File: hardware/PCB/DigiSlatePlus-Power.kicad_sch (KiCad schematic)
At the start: 38 parts, among them J3 +8-24 Volt, J4 Battery, J5 Mains, Q3 FS8205A, U21 LM2596S-ADJ, U22 DW01A, U23 TP4056, U24 KA78M05_TO252, U25 LD1117S33TR_SOT223

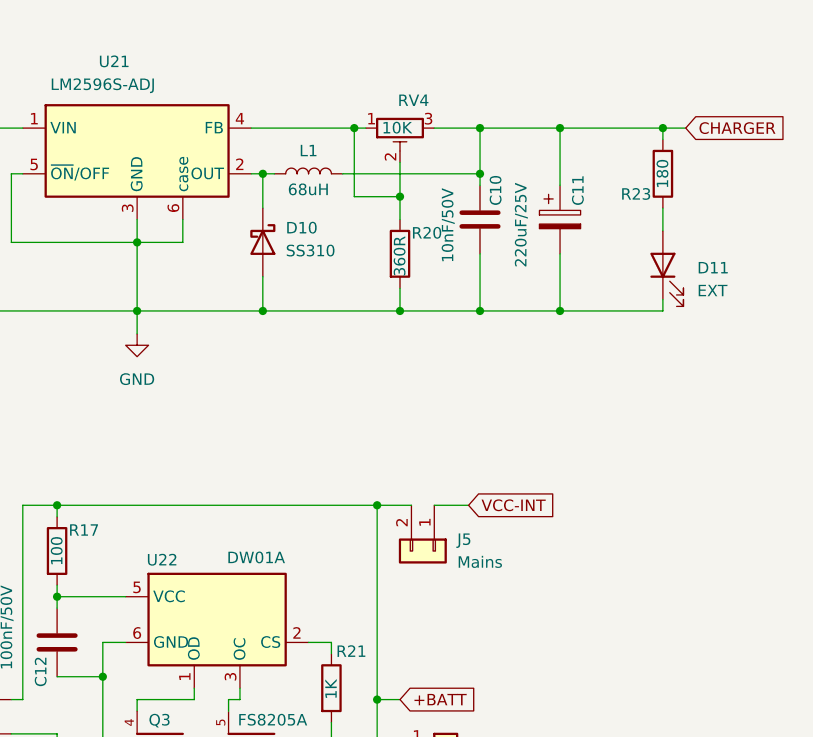
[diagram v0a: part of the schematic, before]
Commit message: final 1.0 board version
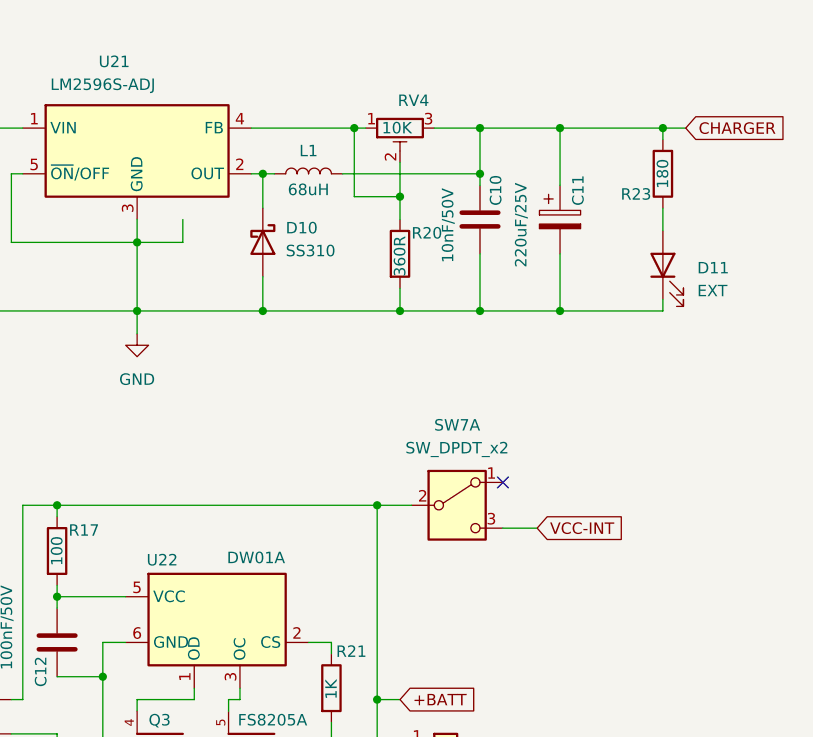
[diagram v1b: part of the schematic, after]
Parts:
- removed J5: Mains, Connector_JST:JST_XH_B2B-XH-AM_1x02_P2.50mm_Vertical, symbol Connector_Generic:Conn_01x02
- added SW7: SW_DPDT_x2, Button_Switch_THT:SW_Slide_SPDT_Angled_CK_OS102011MA1Q, symbol Switch:SW_DPDT_x2
- U21: footprint Package_TO_SOT_SMD:TO-263-5_TabPin6 -> Package_TO_SOT_SMD:TO-263-5_TabPin3
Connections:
- net +BATT: now also SW7.2 (B)
- net GND: no longer U21.6 (case)
- net VCC-INT: now also SW7.3 (C)
- no-connect marks 1 -> 2
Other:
- title: (none) -> DigiSlate+
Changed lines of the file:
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@@
 	(generator_version "8.0")
 	(paper "A4")
+	(title_block
+		(title "DigiSlate+")
+		(date "2024-09-05")
+		(rev "1.0")
+	)
 	(junction
 		(at 228.6 69.85)
@@
 	)
 	(no_connect
+		(at 121.92 109.22)
+	)
+	(no_connect
 		(at 88.9 144.78)
 	)
@@
 	(wire
 		(pts
-			(xy 118.11 111.76) (xy 114.3 111.76)
+			(xy 125.73 114.3) (xy 121.92 114.3)
 		)
 		(stroke
@@
 	(global_label "VCC-INT"
 		(shape input)
-		(at 118.11 111.76 0)
+		(at 125.73 114.3 0)
 		(fields_autoplaced yes)
 		(effects
@@
 		)
 		(property "Intersheetrefs" "${INTERSHEET_REFS}"
-			(at 129.1991 111.76 0)
+			(at 136.8191 114.3 0)
 			(effects
 				(font
@@
 			)
 		)
-		(property "Footprint" "Package_TO_SOT_SMD:TO-263-5_TabPin6"
+		(property "Footprint" "Package_TO_SOT_SMD:TO-263-5_TabPin3"
 			(at 82.55 78.74 0)
 			(effects
@@
 		(pin "2"
 		)
-		(pin "6"
-		)
 		(instances
 			(project "DigiSlatePlus"
@@
 	)
 	(symbol
+		(lib_id "Switch:SW_DPDT_x2")
+		(at 116.84 111.76 0)
+		(unit 1)
+		(exclude_from_sim no)
+		(in_bom yes)
+		(on_board yes)
+		(dnp no)
+		(fields_autoplaced yes)
+		(property "Reference" "SW7"
+			(at 116.84 102.87 0)
+			(effects
+				(font
+					(size 1.27 1.27)
+				)
+			)
+		)
+		(property "Value" "SW_DPDT_x2"
+			(at 116.84 105.41 0)
+			(effects
+				(font
+					(size 1.27 1.27)
+				)
+			)
+		)
+		(property "Footprint" "Button_Switch_THT:SW_Slide_SPDT_Angled_CK_OS102011MA1Q"
+			(at 116.84 111.76 0)
+			(effects
+				(font
+					(size 1.27 1.27)
+				)
+				(hide yes)
+			)
+		)
+		(property "Datasheet" "~"
+			(at 116.84 111.76 0)
+			(effects
+				(font
+					(size 1.27 1.27)
+				)
+				(hide yes)
+			)
+		)
+		(property "Description" "Switch, dual pole double throw, separate symbols"
+			(at 116.84 111.76 0)
+			(effects
+				(font
+					(size 1.27 1.27)
+				)
+				(hide yes)
+			)
+		)
+		(pin "3"
+		)
+		(pin "4"
+		)
+		(pin "5"
+		)
+		(pin "6"
+		)
+		(pin "1"
+		)
+		(pin "2"
+		)
+		(instances
+			(project ""
+				(path "/dcb9cf24-5afa-4bbe-8afa-a00529143e4d/8d8c6cc3-ae5a-4a9a-87ce-71fd40365acc"
+					(reference "SW7")
+					(unit 1)
+				)
+			)
+		)
+	)
+	(symbol
 		(lib_id "Device:C")
 		(at 228.6 121.92 0)
@@
 					(unit 1)
 				)
-			)
-		)
-	)
-	(symbol
-		(lib_id "Connector_Generic:Conn_01x02")
-		(at 114.3 116.84 270)
-		(unit 1)
-		(exclude_from_sim no)
-		(in_bom yes)
-		(on_board yes)
-		(dnp no)
-		(fields_autoplaced yes)
-		(property "Reference" "J5"
-			(at 116.84 115.5699 90)
-			(effects
-				(font
-					(size 1.27 1.27)
-				)
-				(justify left)
-			)
-		)
-		(property "Value" "Mains"
-			(at 116.84 118.1099 90)
-			(effects
-				(font
-					(size 1.27 1.27)
-				)
-				(justify left)
-			)
-		)
-		(property "Footprint" "Connector_JST:JST_XH_B2B-XH-AM_1x02_P2.50mm_Vertical"
-			(at 114.3 116.84 0)
-			(effects
-				(font
-					(size 1.27 1.27)
-				)
-				(hide yes)
-			)
-		)
-		(property "Datasheet" "~"
-			(at 114.3 116.84 0)
-			(effects
-				(font
-					(size 1.27 1.27)
-				)
-				(hide yes)
-			)
-		)
-		(property "Description" "Generic connector, single row, 01x02, script generated (kicad-library-utils/schlib/autogen/connector/)"
-			(at 114.3 116.84 0)
-			(effects
-				(font
-					(size 1.27 1.27)
-				)
-				(hide yes)
-			)
-		)
-		(pin "2"
-		)
-		(pin "1"
-		)
-		(instances
-			(project "DigiSlatePlus"
-				(path "/dcb9cf24-5afa-4bbe-8afa-a00529143e4d/8d8c6cc3-ae5a-4a9a-87ce-71fd40365acc"
-					(reference "J5")
-					(unit 1)
-				)
